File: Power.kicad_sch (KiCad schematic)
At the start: 30 parts, among them U3 LMR51420YDDCR, U4 LM317MDCYR

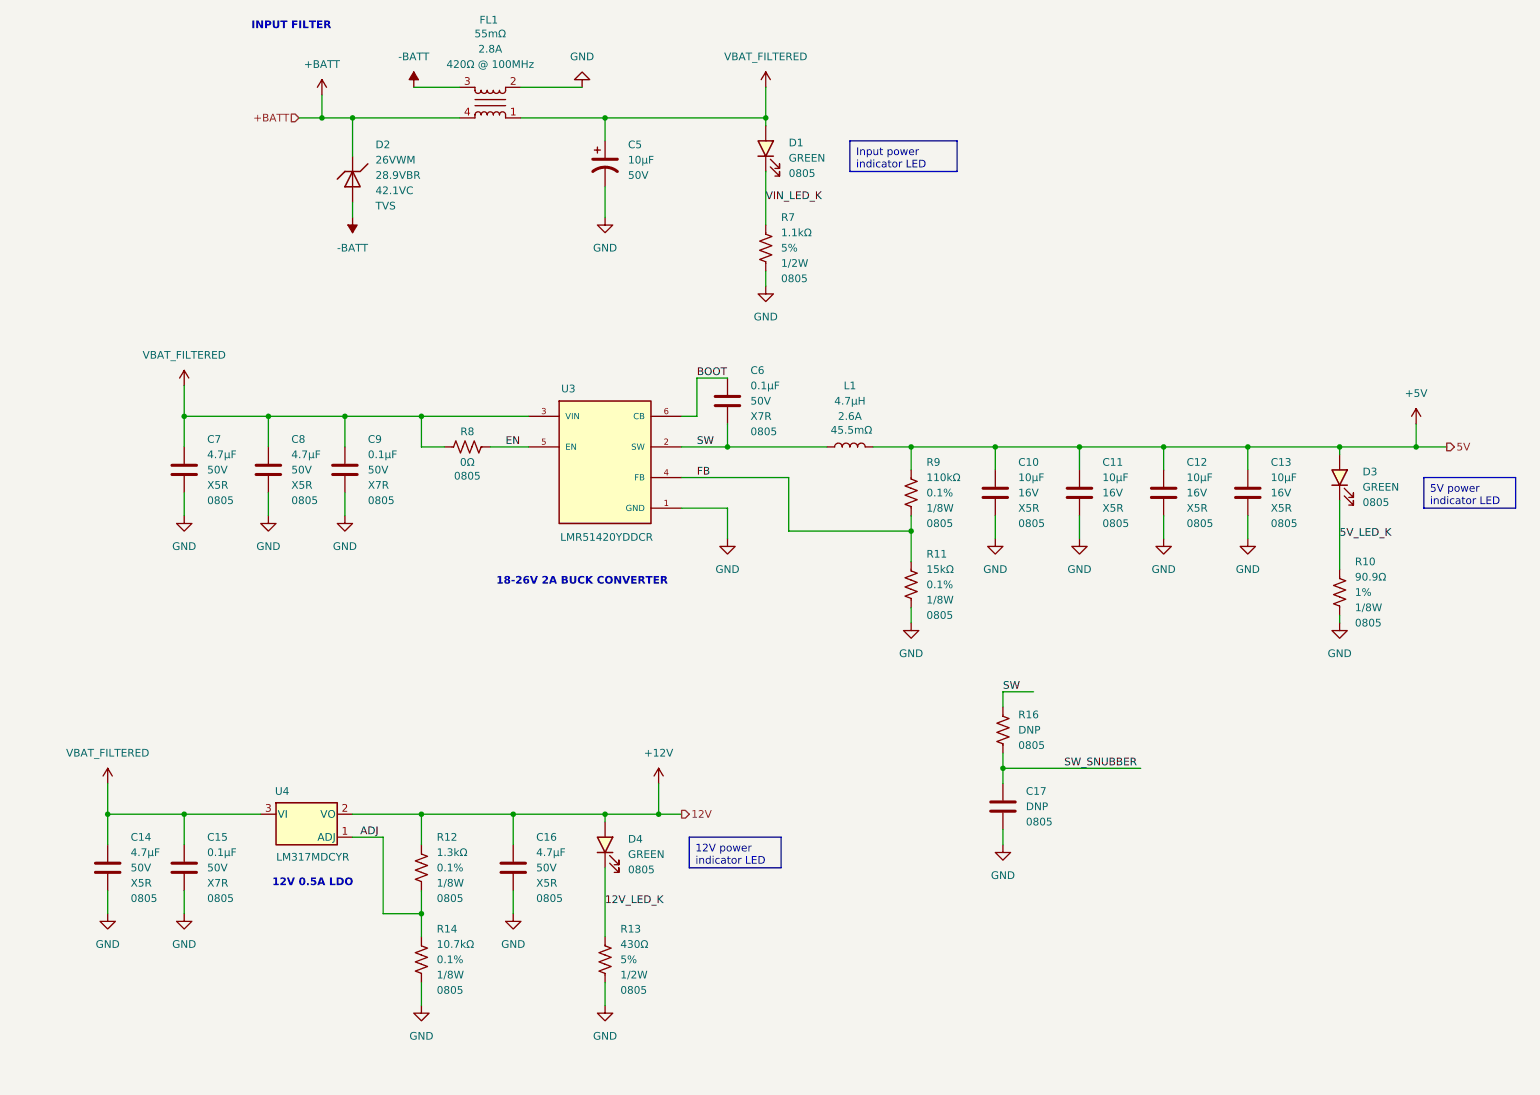
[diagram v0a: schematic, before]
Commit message: 2nd rev is done
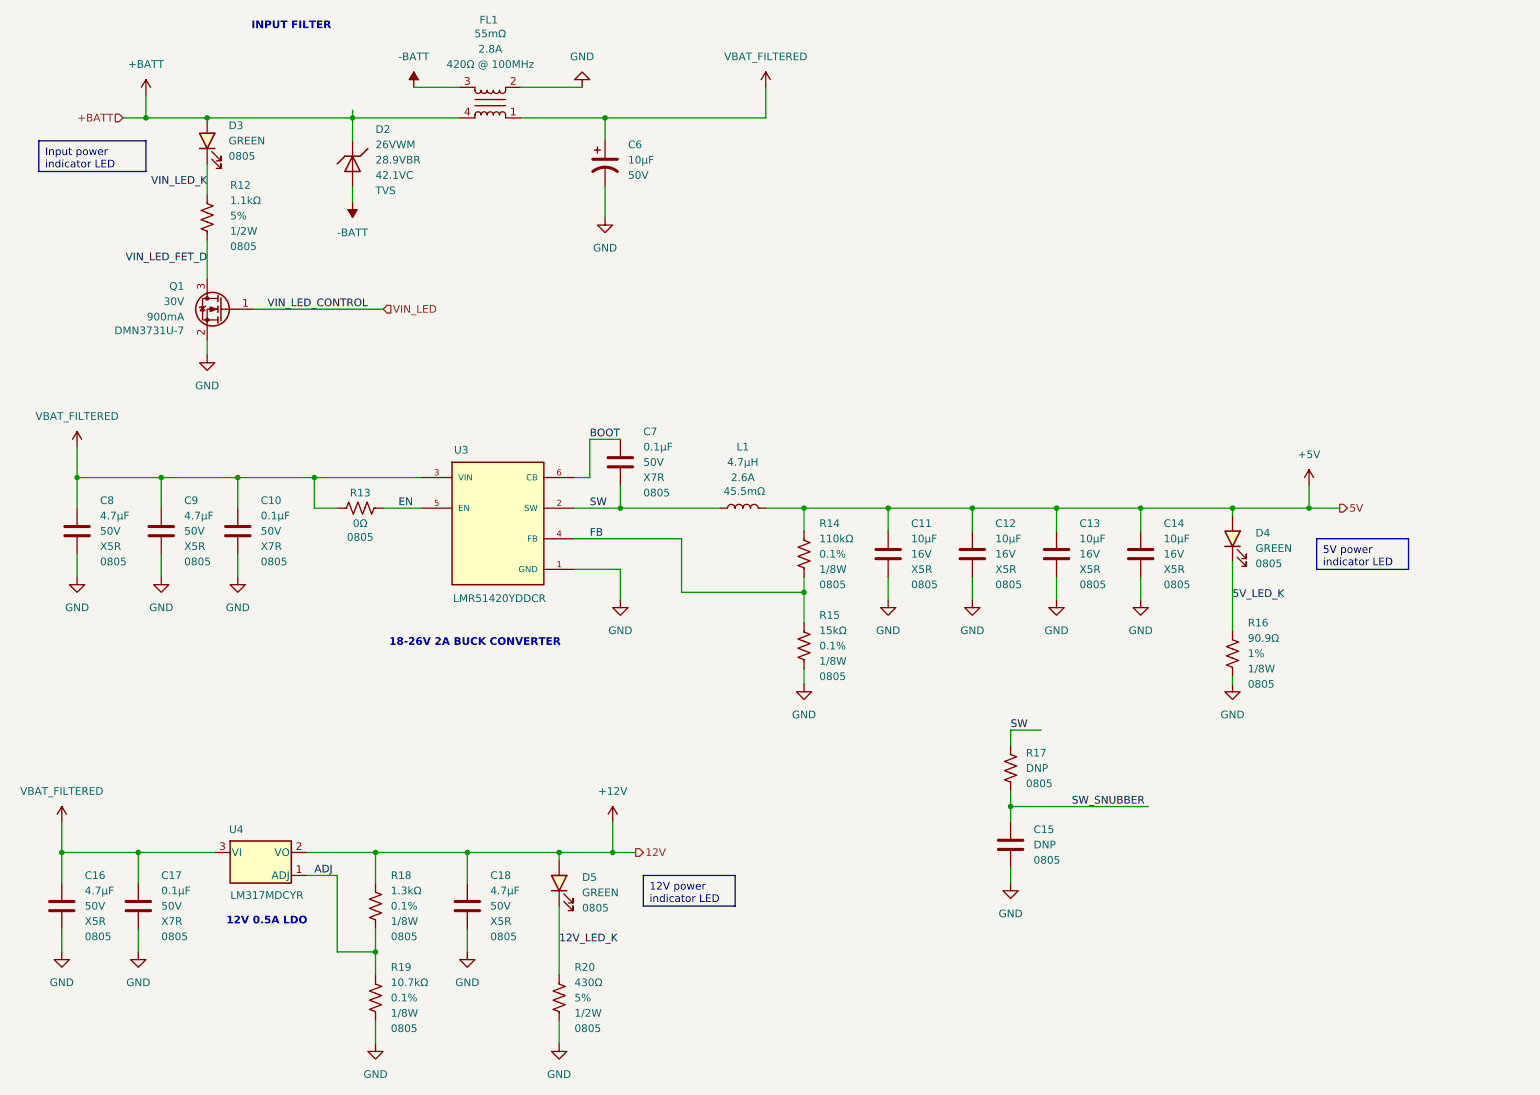
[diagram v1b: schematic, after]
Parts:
- removed D1: 150080GS75000, LED_SMD:LED_0805_2012Metric_Pad1.15x1.40mm_HandSolder, symbol LED:150080GS75000
- removed R7: ERJ-P06J112V, Resistor_SMD:R_0805_2012Metric_Pad1.20x1.40mm_HandSolder, symbol Resistors:ERJ-P06J112V
- added D3: 150080GS75000, LED_SMD:LED_0805_2012Metric_Pad1.15x1.40mm_HandSolder, symbol LED:150080GS75000
- added Q1: DMN3731U-7, Package_TO_SOT_SMD:SOT-23-3_DMN3731U-7, symbol Transistor_FET:DMN3731U-7
- added R12: ERJ-P06J112V, Resistor_SMD:R_0805_2012Metric_Pad1.20x1.40mm_HandSolder, symbol Resistors:ERJ-P06J112V
- renumbered C9 to C10, C10 to C11, C11 to C12, C12 to C13, C13 to C14, C17 to C15, C14 to C16, C15 to C17, C16 to C18, C5 to C6, C6 to C7, C7 to C8, C8 to C9, D3 to D4, D4 to D5, R8 to R13, R9 to R14, R11 to R15, R10 to R16, R16 to R17, R12 to R18, R14 to R19, R13 to R20
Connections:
- net +BATT: now also D3.2 (A)
- net GND: now also Q1.2 (S)
- net VIN_LED_K: now also D3.1 (K), R12.1
- new net VIN_LED: Q1.1 (G)
- new net VIN_LED_FET_D: Q1.3 (D), R12.2
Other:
- moved on the sheet: C10, C11, C12, C13, C14, C15, C16, C17, C18, C7, C8, C9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
